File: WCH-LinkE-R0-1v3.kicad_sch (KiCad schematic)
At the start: 33 parts, among them Q1 IRLML2502TRPBF, Q2 IRLML2502TRPBF, SW1 PTS636_SL43_SMTR_LFS, SW2 PTS636_SL43_SMTR_LFS, SW3 PTS636_SL43_SMTR_LFS, U2 CH32V305FBP6

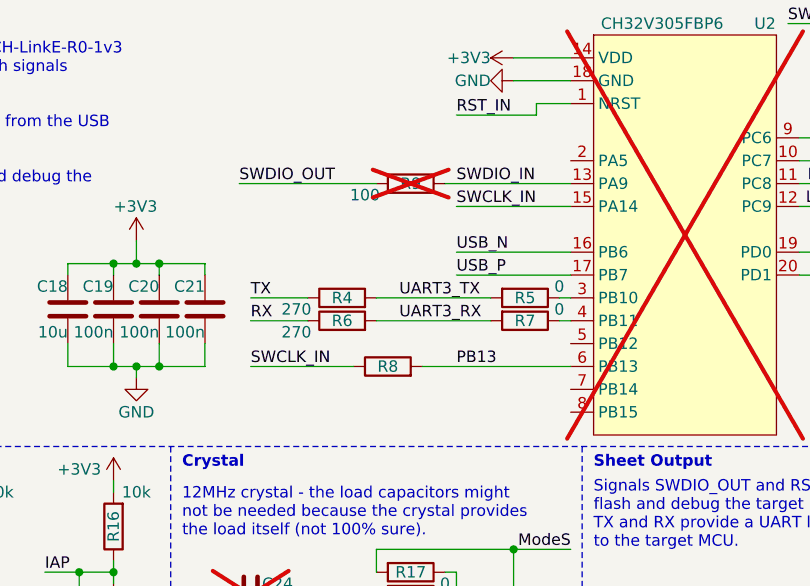
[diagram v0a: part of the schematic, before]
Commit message: Update design
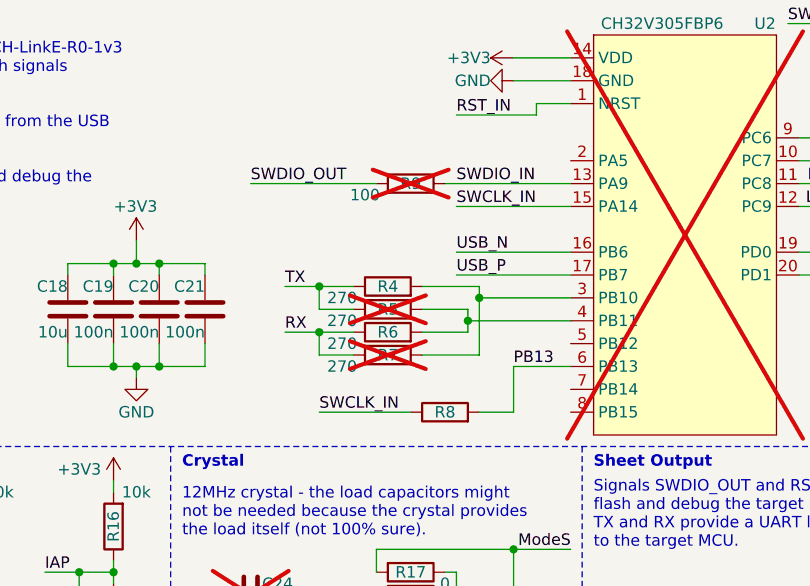
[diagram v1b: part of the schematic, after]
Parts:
- R5, R7: value 0 -> 270; MPN GPR02010R -> GPR0402270R; now not fitted; now left out of the parts list
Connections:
- net RX: now also R7.1
- net TX: now also R5.1
- net at U2.3 (PB10): now also R4.2, R7.2; no longer R5.1
- net at U2.4 (PB11): now also R5.2, R6.2; no longer R7.1
- removed net UART3_RX: R6.2, R7.2
- removed net UART3_TX: R4.2, R5.2
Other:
- moved on the sheet: R4, R6, R8
